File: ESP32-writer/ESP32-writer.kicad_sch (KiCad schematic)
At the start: 12 parts, among them J1 USB2.0_C, J2 UART-OUTPUT, Q1 2N7000, Q2 2N7000, U1 CH340C

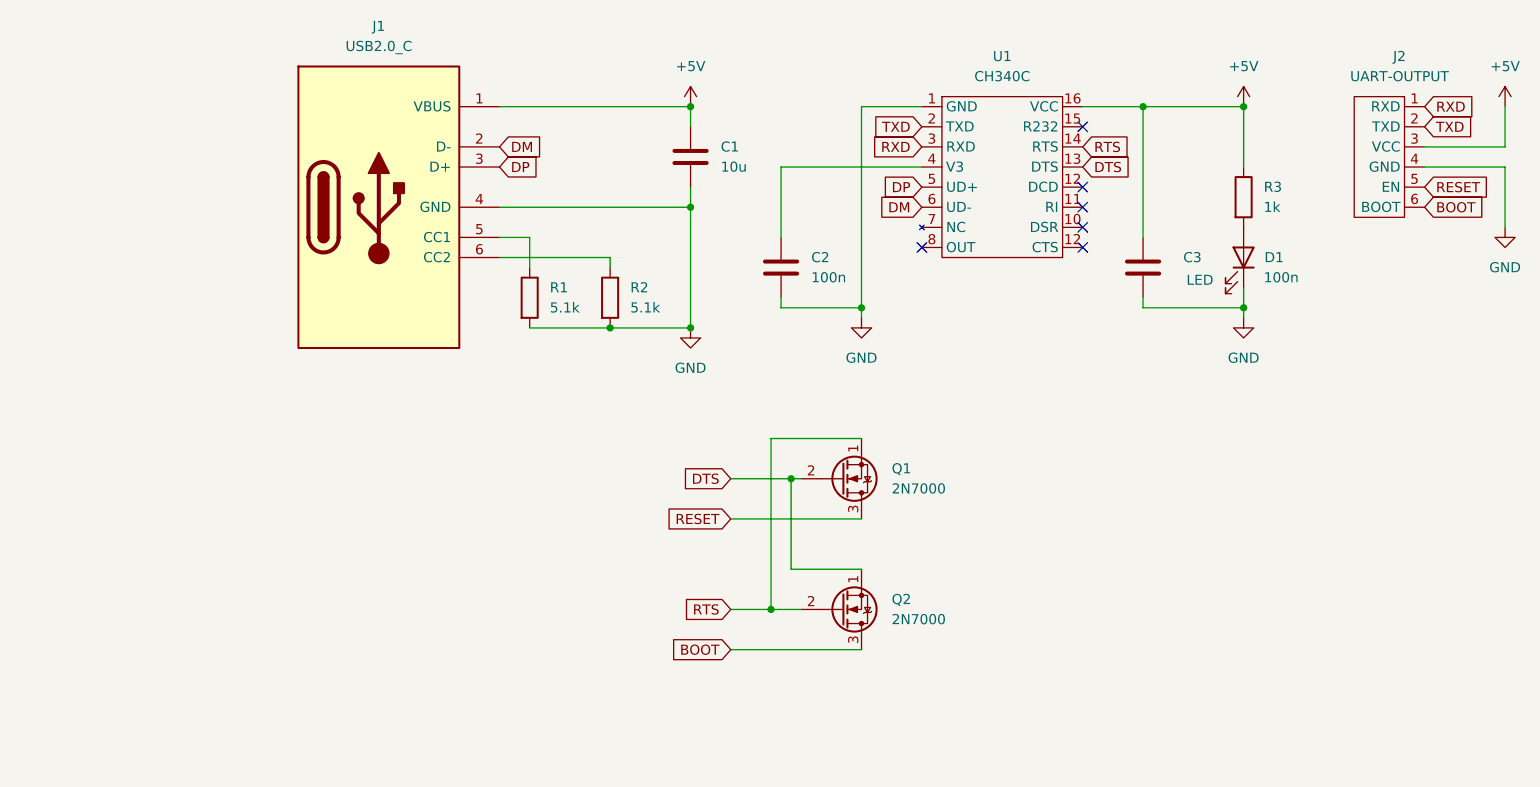
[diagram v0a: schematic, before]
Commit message: esp32-writer
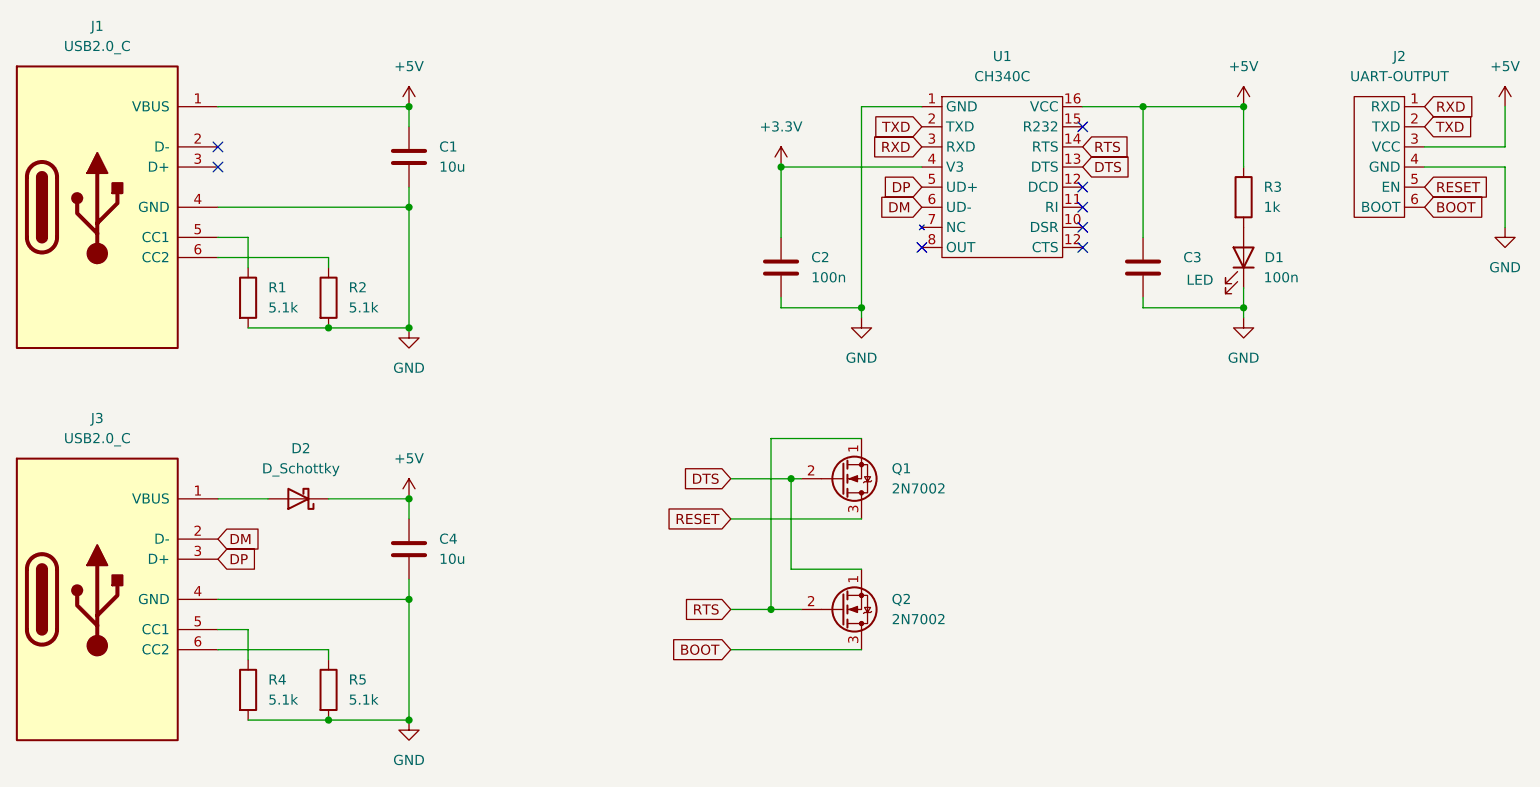
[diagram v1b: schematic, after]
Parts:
- added C4: 10u, $74th:Capacitor_0805_2012, symbol Device:C
- added D2: D_Schottky, $74th:D_SMA, symbol Device:D_Schottky
- added J3: USB2.0_C, $74th:USB-C-12-Pin-MidMount-ali-v4, symbol esp32-dev-board:USB2.0_C
- added R4, R5: 5.1k, $74th:Register_0805_2012, symbol Device:R
- C1, C2, C3: footprint (none) -> $74th:Capacitor_0805_2012
- D1: footprint (none) -> $74th:LED_0805_2012Metric_Pad1.15x1.40mm_HandSolder
- J1: footprint (none) -> $74th:USB-C-12-Pin-MidMount-ali-v4
- J2: footprint (none) -> esp32-dev-board:UART
- Q1, Q2: value 2N7000 -> 2N7002; footprint Package_TO_SOT_THT:TO-92_Inline -> Package_TO_SOT_SMD:SOT-23
- R1, R2, R3: footprint (none) -> $74th:Register_0805_2012
- U1: footprint (none) -> Package_SO:SOP-16_3.9x9.9mm_P1.27mm
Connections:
- net +5V: now also C4.1, D2.1 (K)
- net DM: now also J3.2 (D-); no longer J1.2 (D-)
- net DP: now also J3.3 (D+); no longer J1.3 (D+)
- net GND: now also C4.2, J3.4 (GND), R4.2, R5.2
- net +3V3: now reaches C2.1, U1.4 (V3)
- new net: D2.2 (A), J3.1 (VBUS)
- new net: J3.5 (CC1), R4.1
- new net: J3.6 (CC2), R5.1
- no-connect marks 6 -> 8
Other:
- moved on the sheet: C1, J1, R1, R2
